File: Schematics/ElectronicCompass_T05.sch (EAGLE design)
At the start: 64 parts, among them Q1 FDN360P, Q2 FDN360P, Q3 FDN360P, Q4 FDN360P, Q5 BC817-16LT1SMD, Q6 BC817-16LT1SMD, U1 ATMEGA32U4, X1 USBSMD, Y1 16MHz

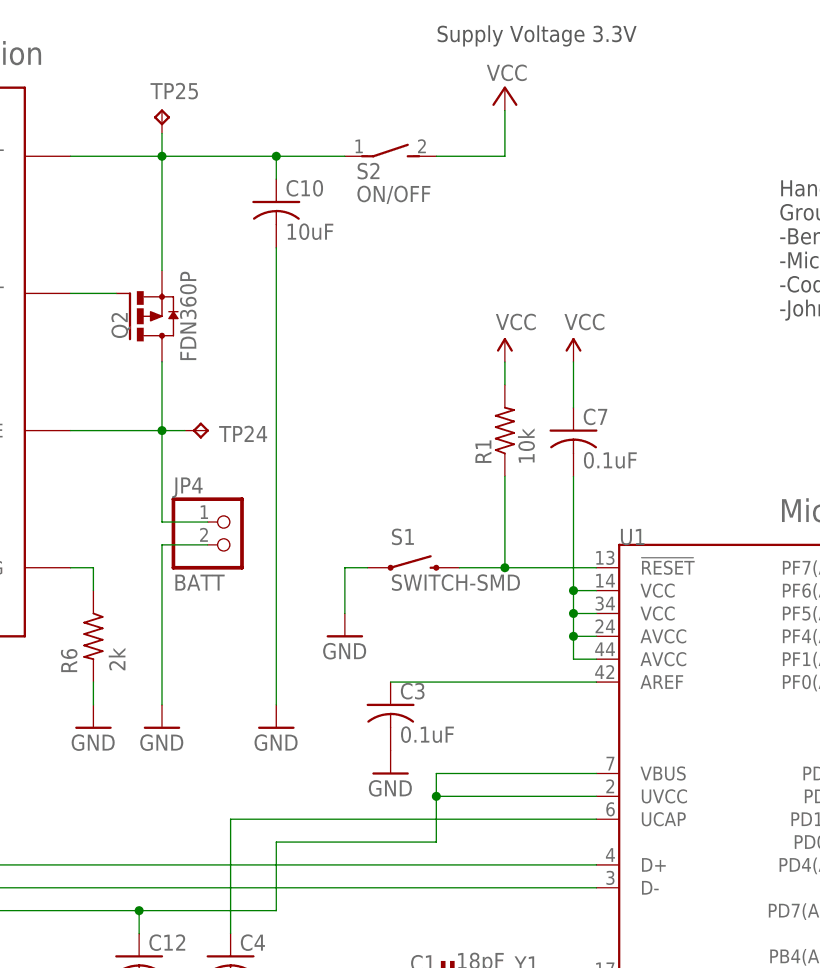
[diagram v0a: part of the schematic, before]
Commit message: sch changes
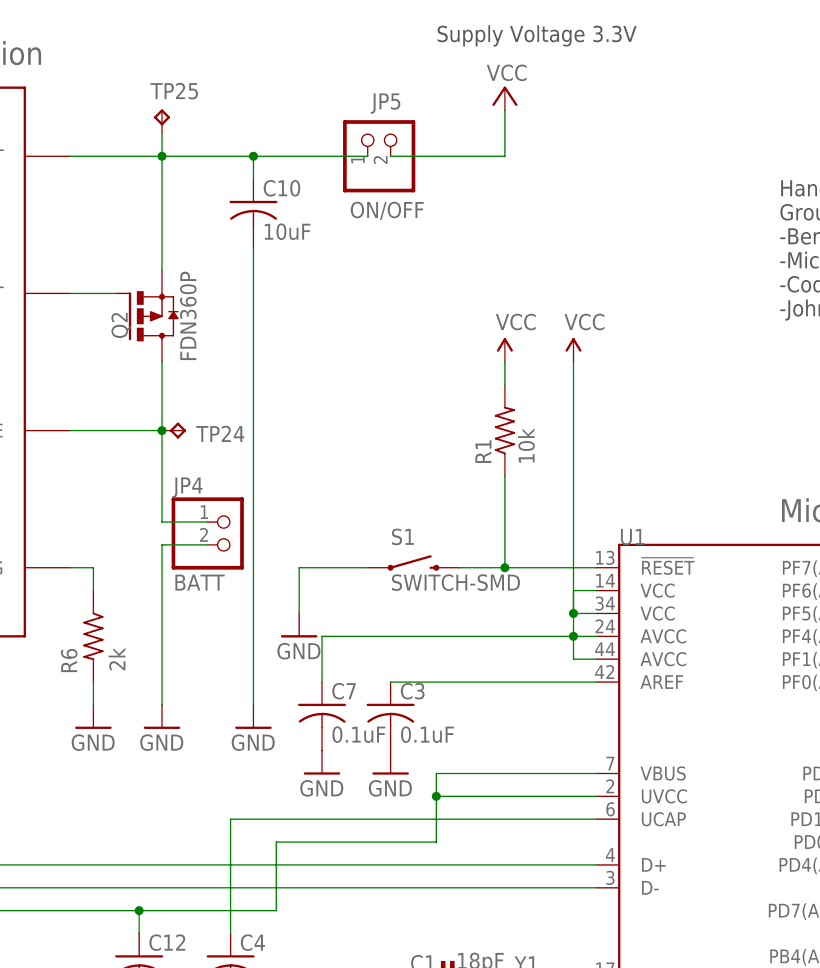
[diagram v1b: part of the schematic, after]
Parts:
- removed S2: ON/OFF, switch-dil:DS01E
- added JP5: ON/OFF, pinhead:PINHD-1X2
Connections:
- removed net N$11: C7.2, U1.AVCC@24, U1.AVCC@44, U1.VCC@14, U1.VCC@34
- net GND: now also C7.2
- net N$36: now also JP5.1; no longer S2.1
- net VCC: now also JP5.2, U1.AVCC@24, U1.AVCC@44, U1.VCC@14, U1.VCC@34; no longer S2.2
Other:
- moved on the sheet: C10, C7, TP24
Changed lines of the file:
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@@
 <part name="TP22" library="testpad" deviceset="TP" device="TP06R"/>
 <part name="TP23" library="testpad" deviceset="TP" device="TP06R"/>
-<part name="S2" library="switch-dil" deviceset="DS01E" device="" value="ON/OFF"/>
 <part name="TP24" library="testpad" deviceset="TP" device="TP06R"/>
 <part name="TP25" library="testpad" deviceset="TP" device="TP06R"/>
@@
 <part name="GND20" library="supply1" deviceset="GND" device=""/>
 <part name="GND21" library="supply1" deviceset="GND" device=""/>
+<part name="JP5" library="pinhead" deviceset="PINHD-1X2" device="" value="ON/OFF"/>
+<part name="GND22" library="SparkFun" deviceset="GND" device=""/>
 </parts>
 <sheets>
@@
 </instance>
 <instance part="S1" gate="G$1" x="106.68" y="22.86"/>
-<instance part="GND1" gate="1" x="99.06" y="15.24"/>
+<instance part="GND1" gate="1" x="93.98" y="15.24"/>
 <instance part="P+1" gate="1" x="116.84" y="45.72" smashed="yes">
 <attribute name="VALUE" x="115.824" y="49.276" size="1.778" layer="96"/>
@@
 </instance>
 <instance part="C5" gate="G$1" x="30.48" y="43.18"/>
-<instance part="C10" gate="G$1" x="91.44" y="63.5"/>
+<instance part="C10" gate="G$1" x="88.9" y="63.5"/>
 <instance part="C11" gate="G$1" x="5.08" y="43.18"/>
-<instance part="GND5" gate="1" x="91.44" y="5.08" smashed="yes">
-<attribute name="VALUE" x="88.9" y="2.54" size="1.778" layer="96"/>
+<instance part="GND5" gate="1" x="88.9" y="5.08" smashed="yes">
+<attribute name="VALUE" x="86.36" y="2.54" size="1.778" layer="96"/>
 </instance>
 <instance part="GND9" gate="1" x="50.8" y="5.08"/>
@@
 <attribute name="TP_SIGNAL_NAME" x="252.73" y="-52.07" size="1.778" layer="97" rot="R90"/>
 </instance>
-<instance part="S2" gate="1" x="104.14" y="68.58" rot="R270"/>
-<instance part="TP24" gate="G$1" x="83.82" y="38.1" smashed="yes" rot="R270">
-<attribute name="NAME" x="85.09" y="36.83" size="1.778" layer="95"/>
-<attribute name="TP_SIGNAL_NAME" x="82.55" y="36.83" size="1.778" layer="97" rot="R270"/>
+<instance part="TP24" gate="G$1" x="81.28" y="38.1" smashed="yes" rot="R270">
+<attribute name="NAME" x="82.55" y="36.83" size="1.778" layer="95"/>
+<attribute name="TP_SIGNAL_NAME" x="80.01" y="36.83" size="1.778" layer="97" rot="R270"/>
 </instance>
 <instance part="TP25" gate="G$1" x="78.74" y="73.66"/>
@@
 <instance part="GND3" gate="1" x="96.52" y="-30.48"/>
 <instance part="GND6" gate="1" x="22.86" y="5.08"/>
-<instance part="C7" gate="G$1" x="124.46" y="38.1"/>
+<instance part="C7" gate="G$1" x="96.52" y="7.62"/>
 <instance part="R7" gate="G$1" x="187.96" y="-53.34" smashed="yes">
 <attribute name="NAME" x="184.15" y="-51.8414" size="1.778" layer="95"/>
@@
 <instance part="GND20" gate="1" x="182.88" y="-78.74"/>
 <instance part="GND21" gate="1" x="187.96" y="-35.56"/>
+<instance part="JP5" gate="G$1" x="104.14" y="71.12" smashed="yes" rot="R90">
+<attribute name="NAME" x="105.41" y="75.565" size="1.778" layer="95" rot="R180"/>
+<attribute name="VALUE" x="107.95" y="63.5" size="1.778" layer="96" rot="R180"/>
+</instance>
+<instance part="GND22" gate="1" x="96.52" y="0"/>
 </instances>
 <busses>
@@
 <net name="GND" class="0">
 <segment>
-<wire x1="99.06" y1="17.78" x2="99.06" y2="22.86" width="0.1524" layer="91"/>
-<wire x1="99.06" y1="22.86" x2="101.6" y2="22.86" width="0.1524" layer="91"/>
+<wire x1="93.98" y1="17.78" x2="93.98" y2="22.86" width="0.1524" layer="91"/>
+<wire x1="93.98" y1="22.86" x2="101.6" y2="22.86" width="0.1524" layer="91"/>
 <pinref part="GND1" gate="1" pin="GND"/>
 <pinref part="S1" gate="G$1" pin="1"/>
@@
 <pinref part="C10" gate="G$1" pin="2"/>
 <pinref part="GND5" gate="1" pin="GND"/>
-<wire x1="91.44" y1="7.62" x2="91.44" y2="58.42" width="0.1524" layer="91"/>
+<wire x1="88.9" y1="7.62" x2="88.9" y2="58.42" width="0.1524" layer="91"/>
 </segment>
 <segment>
@@
 <wire x1="187.96" y1="-30.48" x2="187.96" y2="-33.02" width="0.1524" layer="91"/>
 </segment>
+<segment>
+<pinref part="C7" gate="G$1" pin="2"/>
+<pinref part="GND22" gate="1" pin="GND"/>
+</segment>
 </net>
 <net name="VCC" class="0">
@@
 <pinref part="P+3" gate="VCC" pin="VCC"/>
 <wire x1="116.84" y1="73.66" x2="116.84" y2="68.58" width="0.1524" layer="91"/>
-<pinref part="S2" gate="1" pin="2"/>
-<wire x1="116.84" y1="68.58" x2="109.22" y2="68.58" width="0.1524" layer="91"/>
+<wire x1="116.84" y1="68.58" x2="104.14" y2="68.58" width="0.1524" layer="91"/>
+<pinref part="JP5" gate="G$1" pin="2"/>
 </segment>
 <segment>
@@
 </segment>
 <segment>
-<pinref part="P+2" gate="1" pin="VCC"/>
-<pinref part="C7" gate="G$1" pin="1"/>
-<wire x1="124.46" y1="45.72" x2="124.46" y2="40.64" width="0.1524" layer="91"/>
-</segment>
-<segment>
 <pinref part="P+6" gate="1" pin="VCC"/>
 <pinref part="Q3" gate="G$1" pin="S"/>
@@
 <wire x1="193.04" y1="-53.34" x2="195.58" y2="-53.34" width="0.1524" layer="91"/>
 <junction x="195.58" y="-53.34"/>
+</segment>
+<segment>
+<wire x1="127" y1="20.32" x2="124.46" y2="20.32" width="0.1524" layer="91"/>
+<wire x1="127" y1="17.78" x2="124.46" y2="17.78" width="0.1524" layer="91"/>
+<wire x1="124.46" y1="17.78" x2="124.46" y2="20.32" width="0.1524" layer="91"/>
+<wire x1="127" y1="15.24" x2="124.46" y2="15.24" width="0.1524" layer="91"/>
+<wire x1="124.46" y1="15.24" x2="124.46" y2="17.78" width="0.1524" layer="91"/>
+<wire x1="127" y1="12.7" x2="124.46" y2="12.7" width="0.1524" layer="91"/>
+<wire x1="124.46" y1="12.7" x2="124.46" y2="15.24" width="0.1524" layer="91"/>
+<junction x="124.46" y="17.78"/>
+<junction x="124.46" y="15.24"/>
+<pinref part="U1" gate="G$1" pin="VCC@14"/>
+<pinref part="U1" gate="G$1" pin="VCC@34"/>
+<pinref part="U1" gate="G$1" pin="AVCC@24"/>
+<pinref part="U1" gate="G$1" pin="AVCC@44"/>
+<pinref part="P+2" gate="1" pin="VCC"/>
+<wire x1="124.46" y1="45.72" x2="124.46" y2="17.78" width="0.1524" layer="91"/>
+<pinref part="C7" gate="G$1" pin="1"/>
+<wire x1="124.46" y1="15.24" x2="96.52" y2="15.24" width="0.1524" layer="91"/>
+<wire x1="96.52" y1="15.24" x2="96.52" y2="10.16" width="0.1524" layer="91"/>
 </segment>
 </net>
@@
 <wire x1="68.58" y1="38.1" x2="78.74" y2="38.1" width="0.1524" layer="91"/>
 <pinref part="TP24" gate="G$1" pin="TP"/>
-<wire x1="78.74" y1="38.1" x2="81.28" y2="38.1" width="0.1524" layer="91"/>
 <pinref part="Q2" gate="G$1" pin="D"/>
 <wire x1="78.74" y1="38.1" x2="78.74" y2="45.72" width="0.1524" layer="91"/>
@@
 <wire x1="68.58" y1="68.58" x2="78.74" y2="68.58" width="0.1524" layer="91"/>
 <junction x="78.74" y="68.58"/>
-<pinref part="S2" gate="1" pin="1"/>
-<wire x1="99.06" y1="68.58" x2="91.44" y2="68.58" width="0.1524" layer="91"/>
+<wire x1="101.6" y1="68.58" x2="88.9" y2="68.58" width="0.1524" layer="91"/>
 <pinref part="C10" gate="G$1" pin="1"/>
-<wire x1="91.44" y1="68.58" x2="78.74" y2="68.58" width="0.1524" layer="91"/>
-<wire x1="91.44" y1="66.04" x2="91.44" y2="68.58" width="0.1524" layer="91"/>
-<junction x="91.44" y="68.58"/>
+<wire x1="88.9" y1="68.58" x2="78.74" y2="68.58" width="0.1524" layer="91"/>
+<wire x1="88.9" y1="66.04" x2="88.9" y2="68.58" width="0.1524" layer="91"/>
+<junction x="88.9" y="68.58"/>
 <pinref part="U$1" gate="G$1" pin="OUT"/>
+<pinref part="JP5" gate="G$1" pin="1"/>
 </segment>
 </net>
@@
 </segment>
 </net>
-<net name="N$11" class="0">
-<segment>
-<wire x1="127" y1="20.32" x2="124.46" y2="20.32" width="0.1524" layer="91"/>
-<wire x1="127" y1="17.78" x2="124.46" y2="17.78" width="0.1524" layer="91"/>
-<wire x1="124.46" y1="17.78" x2="124.46" y2="20.32" width="0.1524" layer="91"/>
-<wire x1="127" y1="15.24" x2="124.46" y2="15.24" width="0.1524" layer="91"/>
-<wire x1="124.46" y1="15.24" x2="124.46" y2="17.78" width="0.1524" layer="91"/>
-<wire x1="127" y1="12.7" x2="124.46" y2="12.7" width="0.1524" layer="91"/>
-<wire x1="124.46" y1="12.7" x2="124.46" y2="15.24" width="0.1524" layer="91"/>
-<junction x="124.46" y="17.78"/>
-<junction x="124.46" y="15.24"/>
-<pinref part="U1" gate="G$1" pin="VCC@14"/>
-<pinref part="U1" gate="G$1" pin="VCC@34"/>
-<pinref part="U1" gate="G$1" pin="AVCC@24"/>
-<pinref part="U1" gate="G$1" pin="AVCC@44"/>
-<pinref part="C7" gate="G$1" pin="2"/>
-<wire x1="124.46" y1="33.02" x2="124.46" y2="20.32" width="0.1524" layer="91"/>
-<junction x="124.46" y="20.32"/>
-</segment>
-</net>
